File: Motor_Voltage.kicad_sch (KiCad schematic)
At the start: 15 parts, among them IC4 AMC1350DWVR

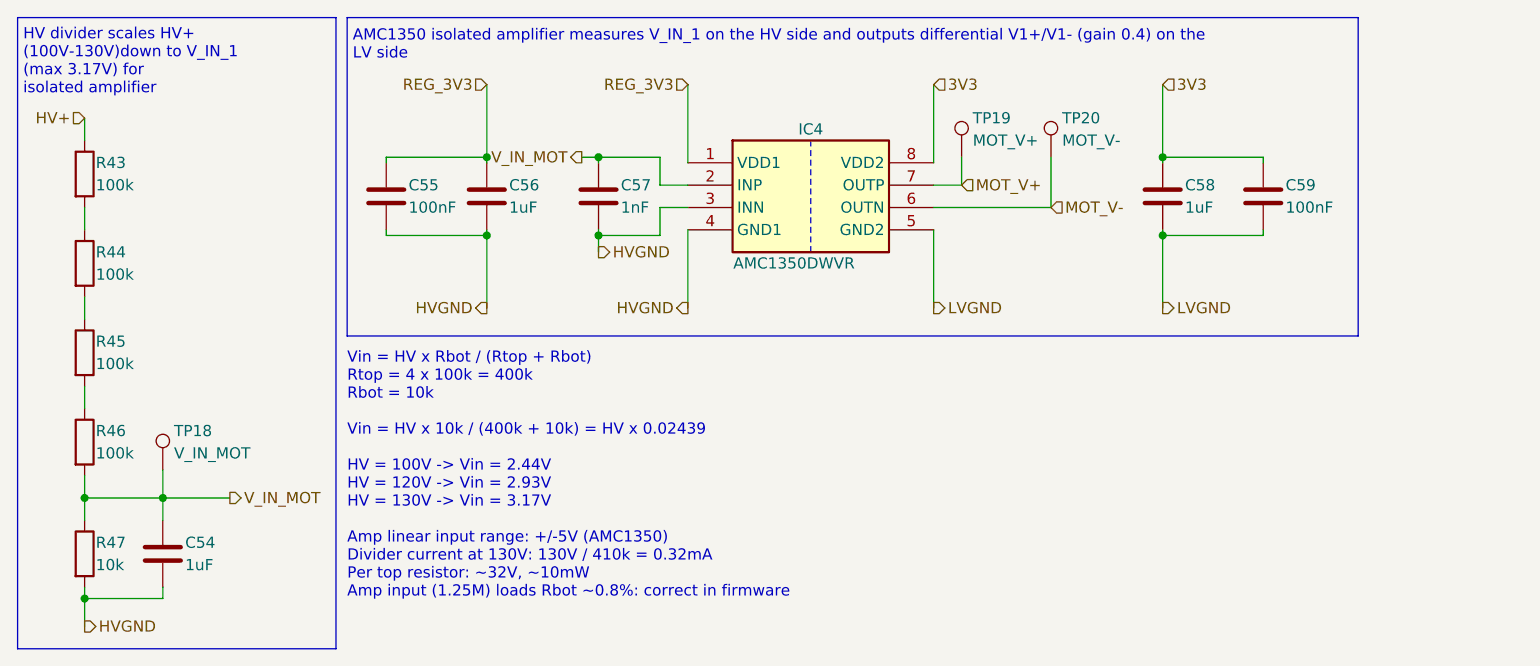
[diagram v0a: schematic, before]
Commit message: shifted hierarchical sheets
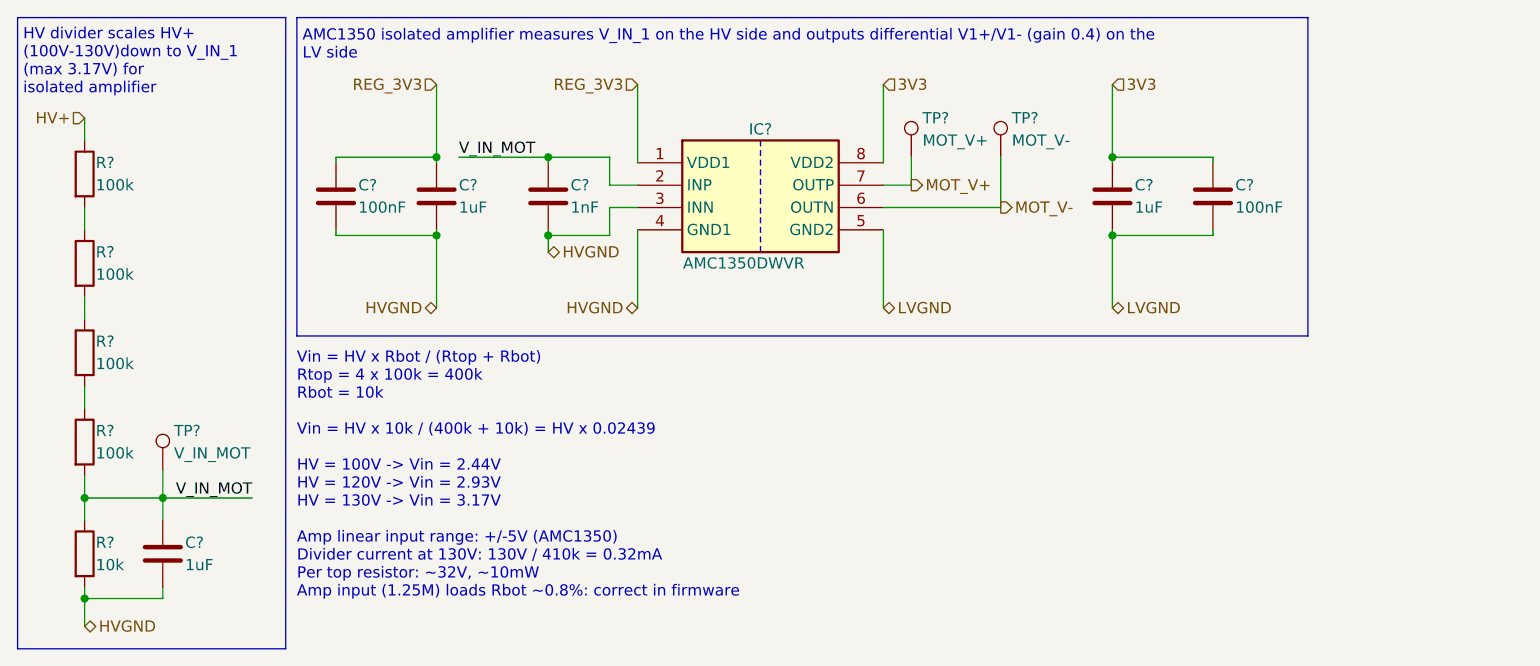
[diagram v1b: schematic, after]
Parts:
- renumbered C56 to C?, C57 to C?, C54 to C?, C58 to C?, C59 to C?, C55 to C?, IC4 to IC?, R47 to R?, R43 to R?, R45 to R?, R46 to R?, R44 to R?, TP18 to TP?, TP20 to TP?, TP19 to TP?
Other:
- moved on the sheet: C?, IC?, TP?
